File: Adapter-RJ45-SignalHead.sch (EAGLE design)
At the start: 4 parts, among them CON1 CONNECTOR-GROVE-4P-2.0-347013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, CON2 CONNECTOR-GROVE-4P-2.0-347013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

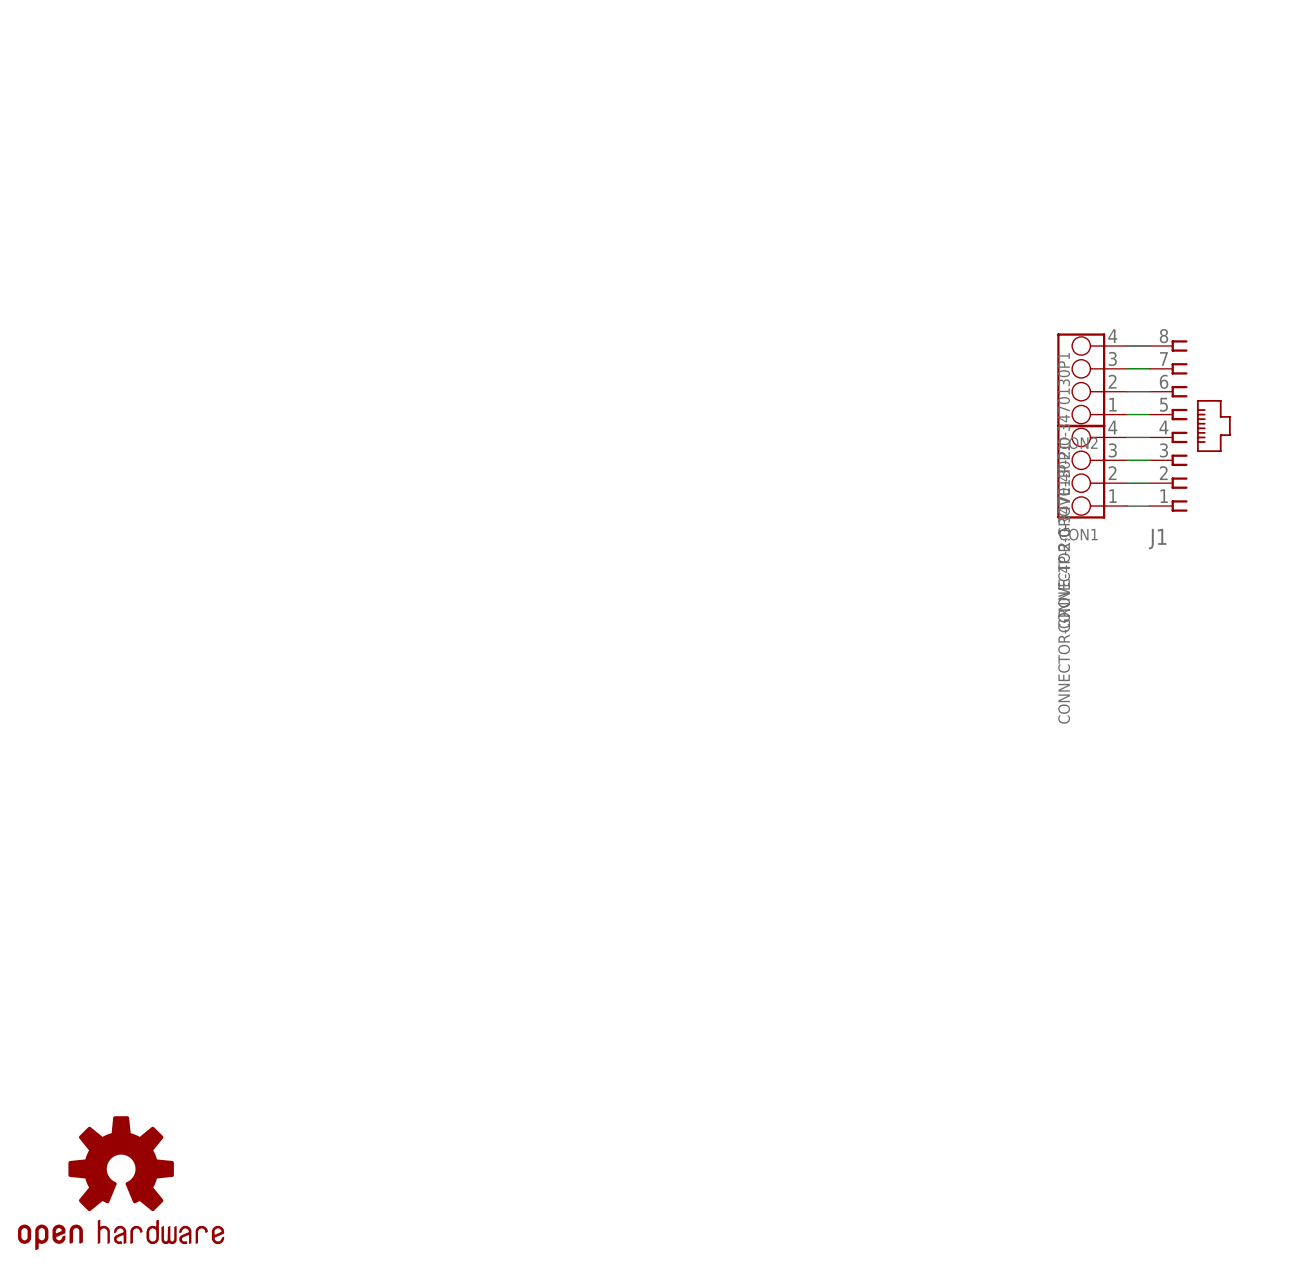
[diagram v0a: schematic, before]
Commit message: V3.2 - added CUT-R
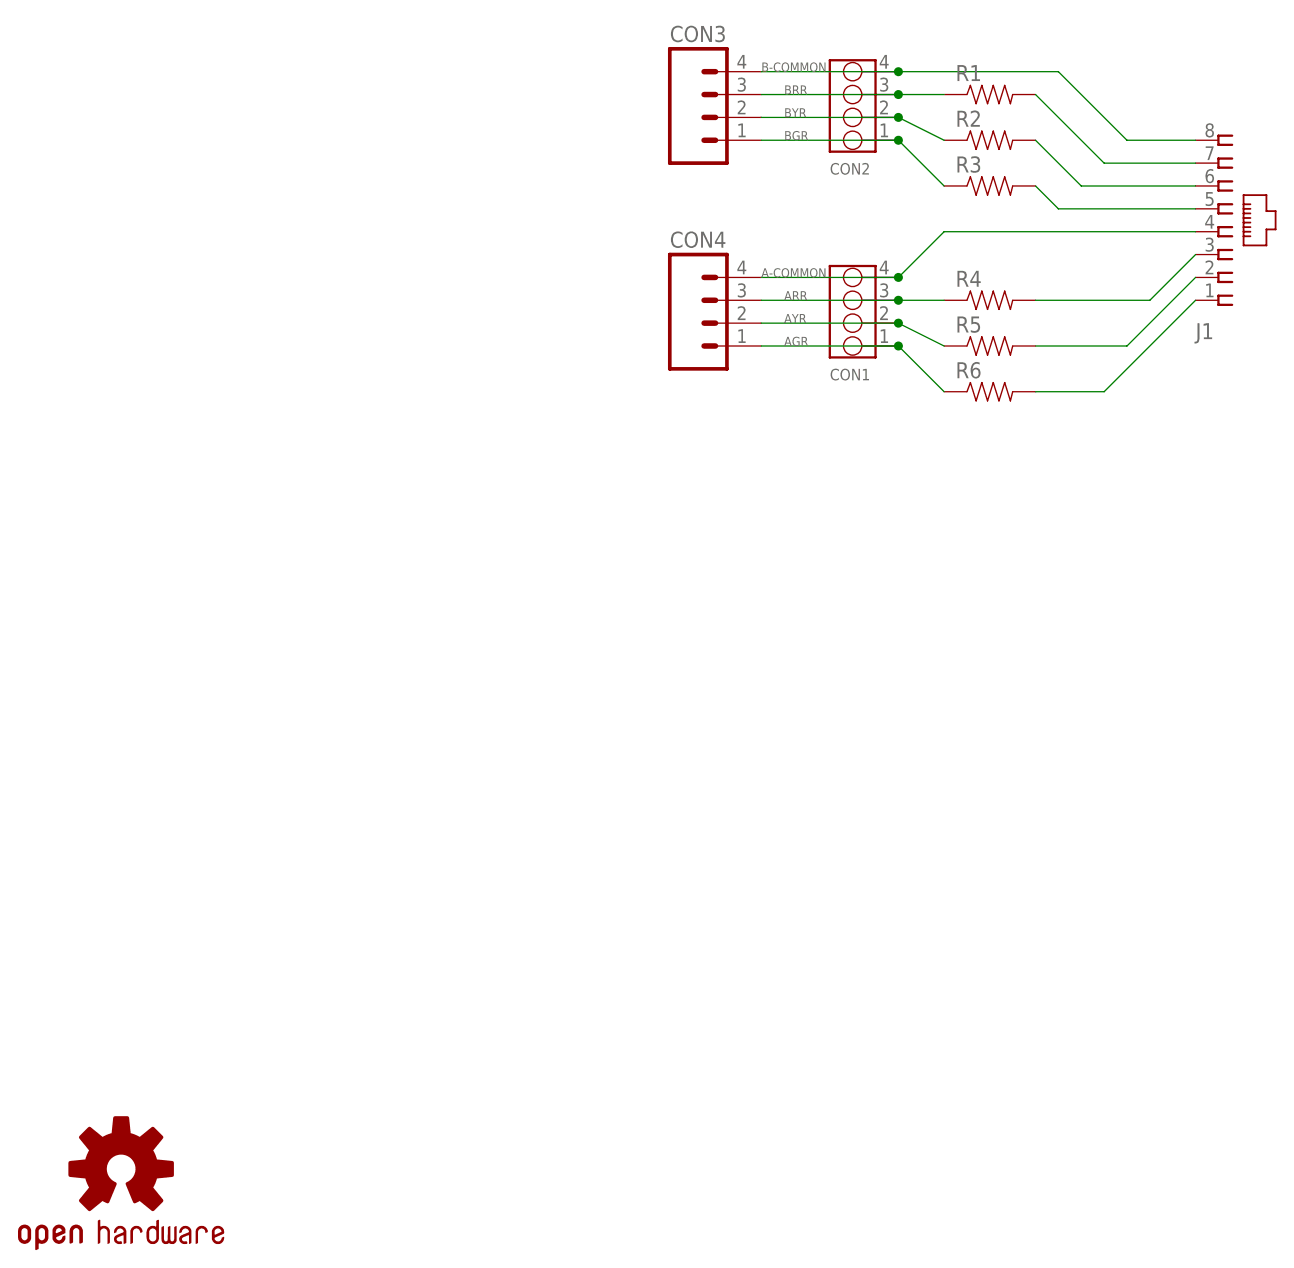
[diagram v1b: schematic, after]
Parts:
- added CON3, CON4: (no value), SPCoast:CONNECTOR-M04LOCK
- added R1, R2, R3, R4, R5, R6: (no value), SPCoast:RPTH-R0
- CON1, CON2: value CONNECTOR-GROVE-4P-2.0-3470130P1 -> (none)
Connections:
- removed net L5: CON2.1, J1.5
- removed net L6: CON2.2, J1.6
- removed net L7: CON2.3, J1.7
- removed net L8: CON2.4, J1.8
- removed net N$1: CON1.1, J1.1
- removed net N$2: CON1.2, J1.2
- removed net N$3: CON1.3, J1.3
- removed net N$4: CON1.4, J1.4
- new net A-COMMON: CON1.4, CON4.4, J1.4
- new net AG: J1.1, R6.2
- new net AGR: CON1.1, CON4.1, R6.1
- new net AR: J1.3, R4.2
- new net ARR: CON1.3, CON4.3, R4.1
- new net AY: J1.2, R5.2
- new net AYR: CON1.2, CON4.2, R5.1
- new net B-COMMON: CON2.4, CON3.4, J1.8
- new net BG: J1.5, R3.2
- new net BGR: CON2.1, CON3.1, R3.1
- new net BR: J1.7, R1.2
- new net BRR: CON2.3, CON3.3, R1.1
- new net BY: J1.6, R2.2
- new net BYR: CON2.2, CON3.2, R2.1
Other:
- note added: "2x 2mm 4-pin"
- note added: "Signal Head Breakout"
- note added: "v3.2"
- note added: "w/ optional resistors"
- note removed: "CMRI Breakout"
- note removed: "RJ45 adapter"
- note removed: "v3.1"
- moved on the sheet: CON1, CON2, J1
